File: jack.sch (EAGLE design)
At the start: 30 parts, among them IC1 NUF2221W1T2G, IC2 ATSAMD21G18, IC3 LDO, SW1 SPST3.5X6MM, X1 TSX-3225 24.0000MF10Z-C3

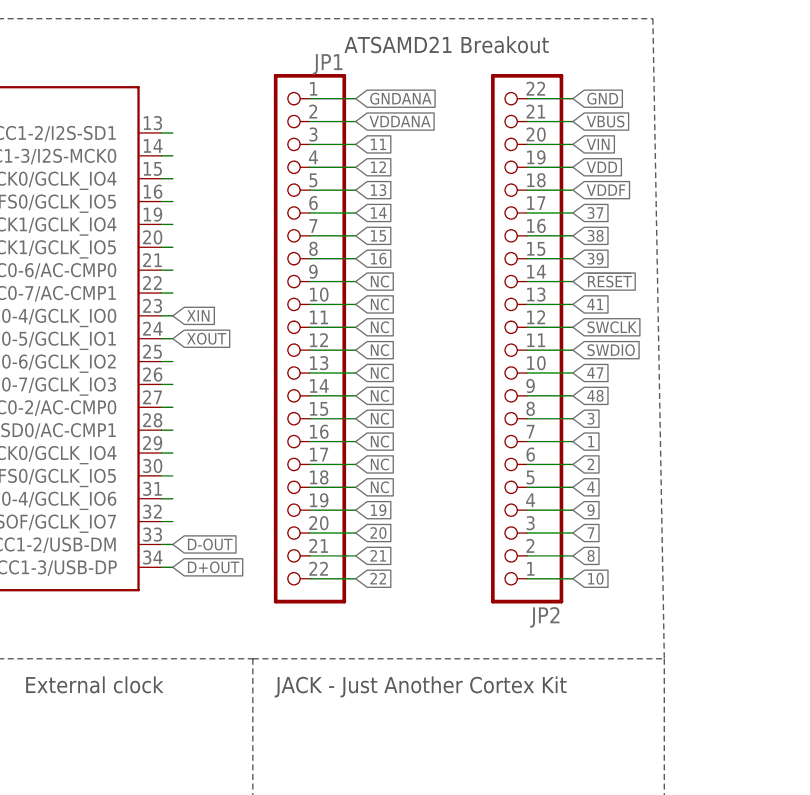
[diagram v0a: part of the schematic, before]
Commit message: :feelsgood: Layout finished!
Minor details gotta be worked now (polishing pours layout)
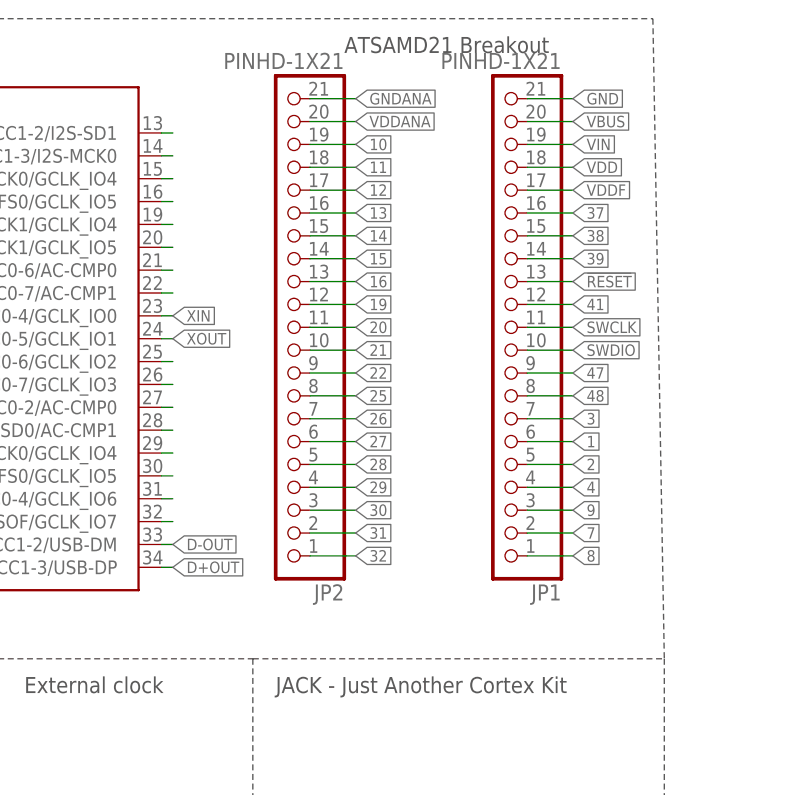
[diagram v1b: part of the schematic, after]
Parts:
- JP1, JP2: value (none) -> PINHD-1X21; device pinhead:PINHD-1X22 -> jack:PINHD-1X21
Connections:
- removed net NC: JP1.10, JP1.11, JP1.12, JP1.13, JP1.14, JP1.15, JP1.16, JP1.17, JP1.18, JP1.9
- net !RESET: now also JP1.13; no longer JP2.14
- net 1: now also JP1.6; no longer JP2.7
- net 10: now also JP2.19; no longer JP2.1
- net 11: now also JP2.18; no longer JP1.3
- net 12: now also JP2.17; no longer JP1.4
- net 13: now also JP2.16; no longer JP1.5
- net 14: now also JP2.15; no longer JP1.6
- net 15: now also JP2.14; no longer JP1.7
- net 16: now also JP2.13; no longer JP1.8
- net 19: now also JP2.12; no longer JP1.19
- net 2: now also JP1.5; no longer JP2.6
- net 20: now also JP2.11; no longer JP1.20
- net 21: now also JP2.10; no longer JP1.21
- net 22: now also JP2.9; no longer JP1.22
- net 25: now also JP2.8
- net 26: now also JP2.7
- net 27: now also JP2.6
- net 28: now also JP2.5
- net 29: now also JP2.4
- net 3: now also JP1.7; no longer JP2.8
- net 30: now also JP2.3
- net 31: now also JP2.2
- net 32: now also JP2.1
- net 37: now also JP1.16; no longer JP2.17
- net 38: now also JP1.15; no longer JP2.16
- net 39: now also JP1.14; no longer JP2.15
- net 4: now also JP1.4; no longer JP2.5
- net 41: now also JP1.12; no longer JP2.13
- net 47: now also JP1.9; no longer JP2.10
- net 48: now also JP1.8; no longer JP2.9
- net 7: now also JP1.2; no longer JP2.3
- net 8: now also JP1.1; no longer JP2.2
- net 9: now also JP1.3; no longer JP2.4
- net GND: now also JP1.21; no longer JP2.22
- net GNDANA: now also JP2.21; no longer JP1.1
- net SWCLK: now also JP1.11; no longer JP2.12
- net SWDIO: now also JP1.10; no longer JP2.11
- net VBUS: now also JP1.20; no longer JP2.21
- net VDD: now also JP1.18; no longer JP2.19
- net VDDANA: now also JP2.20; no longer JP1.2
- net VDDF: now also JP1.17; no longer JP2.18
- net VIN: now also JP1.19; no longer JP2.20
